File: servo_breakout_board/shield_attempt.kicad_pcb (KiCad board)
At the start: 2 copper layers, 74.9 x 44.5 mm, 18 parts

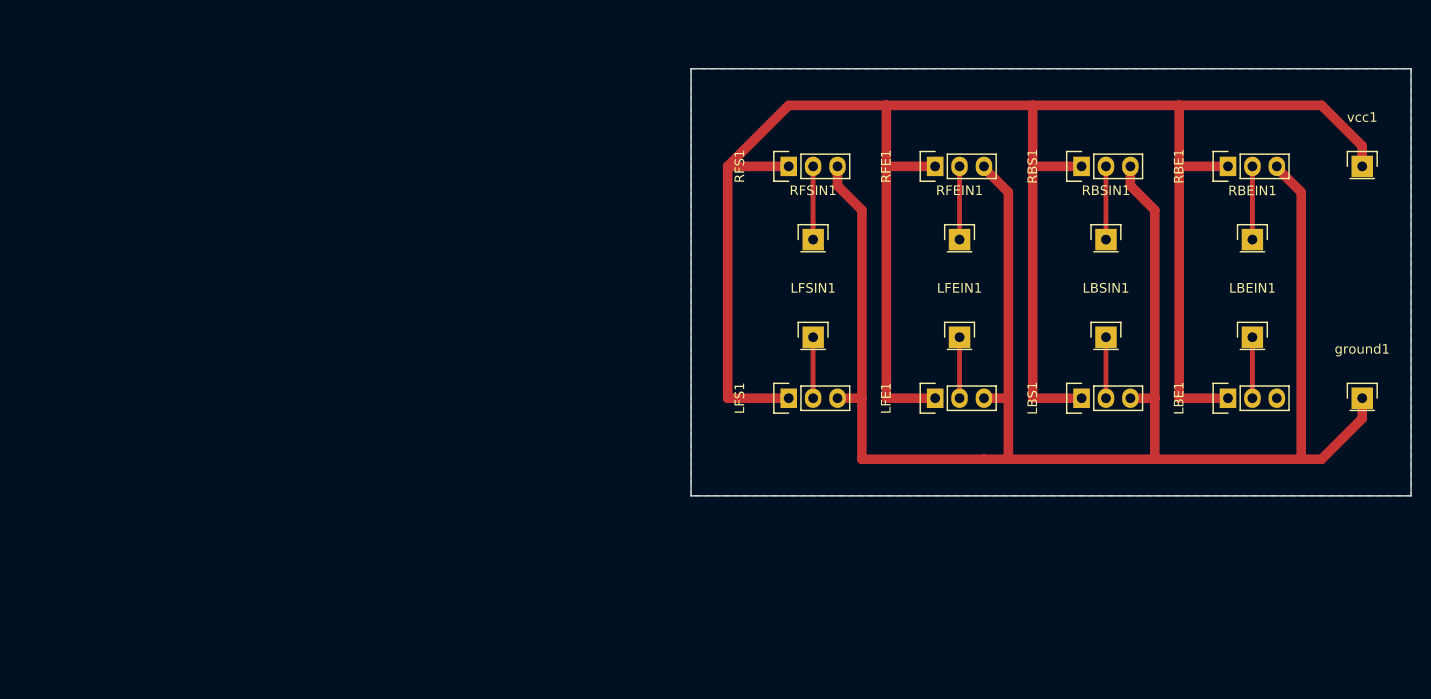
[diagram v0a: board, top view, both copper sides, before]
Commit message: Second attempt at the main board
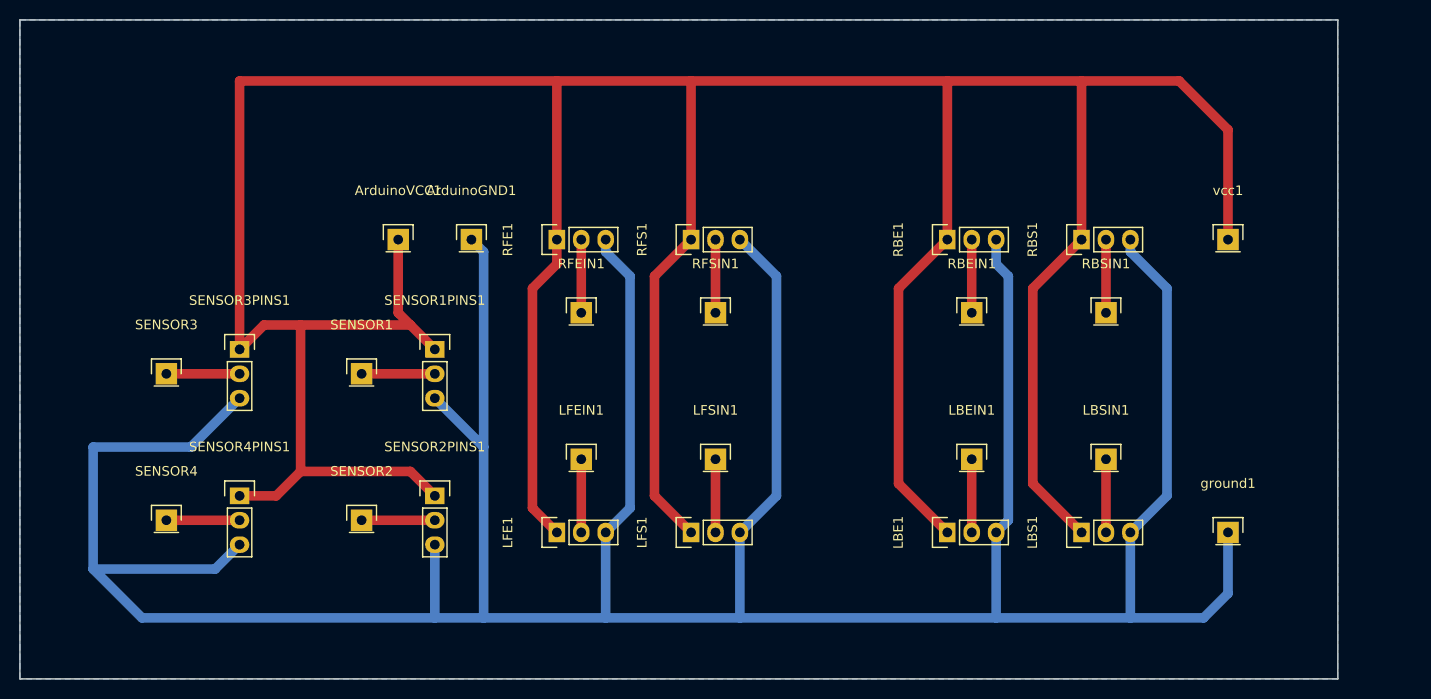
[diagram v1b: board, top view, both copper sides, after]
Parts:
- added ArduinoGND1: CONN_01X01, Pin_Headers:Pin_Header_Straight_1x01, F.Cu at (123.2, 95.2)
- added ArduinoVCC1: CONN_01X01, Pin_Headers:Pin_Header_Straight_1x01, F.Cu at (115.6, 95.2)
- added SENSOR1: CONN_01X01, Pin_Headers:Pin_Header_Straight_1x01, F.Cu at (111.8, 109.2)
- added SENSOR1PINS1: CONN_01X03, Pin_Headers:Pin_Header_Straight_1x03, F.Cu at (119.4, 106.7)
- added SENSOR2: CONN_01X01, Pin_Headers:Pin_Header_Straight_1x01, F.Cu at (111.8, 124.5)
- added SENSOR2PINS1: CONN_01X03, Pin_Headers:Pin_Header_Straight_1x03, F.Cu at (119.4, 121.9)
- added SENSOR3: CONN_01X01, Pin_Headers:Pin_Header_Straight_1x01, F.Cu at (91.4, 109.2)
- added SENSOR3PINS1: CONN_01X03, Pin_Headers:Pin_Header_Straight_1x03, F.Cu at (99.1, 106.7)
- added SENSOR4: CONN_01X01, Pin_Headers:Pin_Header_Straight_1x01, F.Cu at (91.4, 124.5)
- added SENSOR4PINS1: CONN_01X03, Pin_Headers:Pin_Header_Straight_1x03, F.Cu at (99.1, 121.9)
- moved LFE1 41.8 mm to (132.1, 125.7)
- moved LFEIN1 41.4 mm to (134.6, 118.1)
- moved RFEIN1 40.1 mm to (134.6, 102.9)
- moved RFE1 40.1 mm to (132.1, 95.2)
- moved LBE1 32.4 mm to (172.7, 125.7)
- moved LBEIN1 31.9 mm to (175.3, 118.1)
- moved RBE1 30.2 mm to (172.7, 95.2)
- moved RBEIN1 30.2 mm to (175.3, 102.9)
- moved ground1 19.8 mm to (201.9, 125.7)
- moved LFS1 17.3 mm to (146.1, 125.7)
- moved LFSIN1 16.3 mm to (148.6, 118.1)
- moved vcc1 15.9 mm to (201.9, 95.2)
- moved LBS1 14.0 mm to (186.7, 125.7)
- moved LBSIN1 12.7 mm to (189.2, 118.1)
- moved RFS1 12.7 mm to (146.1, 95.2)
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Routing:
- net GND: track 191.1 -> 395.6 mm
- net +5V: track 231.3 -> 415.5 mm
- net Net-(SENSOR4-Pad1): track 0.00 -> 7.62 mm
- net Net-(SENSOR3-Pad1): track 0.00 -> 7.62 mm
- net Net-(SENSOR2-Pad1): track 0.00 -> 7.62 mm
- net Net-(SENSOR1-Pad1): track 0.00 -> 7.62 mm
- net Net-(RFS1-Pad2): track 8.99 -> 7.62 mm
- net Net-(LFS1-Pad2): track 6.35 -> 7.62 mm
- net Net-(LFE1-Pad2): track 6.35 -> 7.62 mm
- net Net-(LBS1-Pad2): track 6.35 -> 7.62 mm
- net Net-(LBE1-Pad2): track 6.35 -> 7.62 mm
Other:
- board size 74.9 x 44.5 mm -> 137.2 x 68.6 mm
